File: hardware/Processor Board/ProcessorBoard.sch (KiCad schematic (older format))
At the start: 0 parts

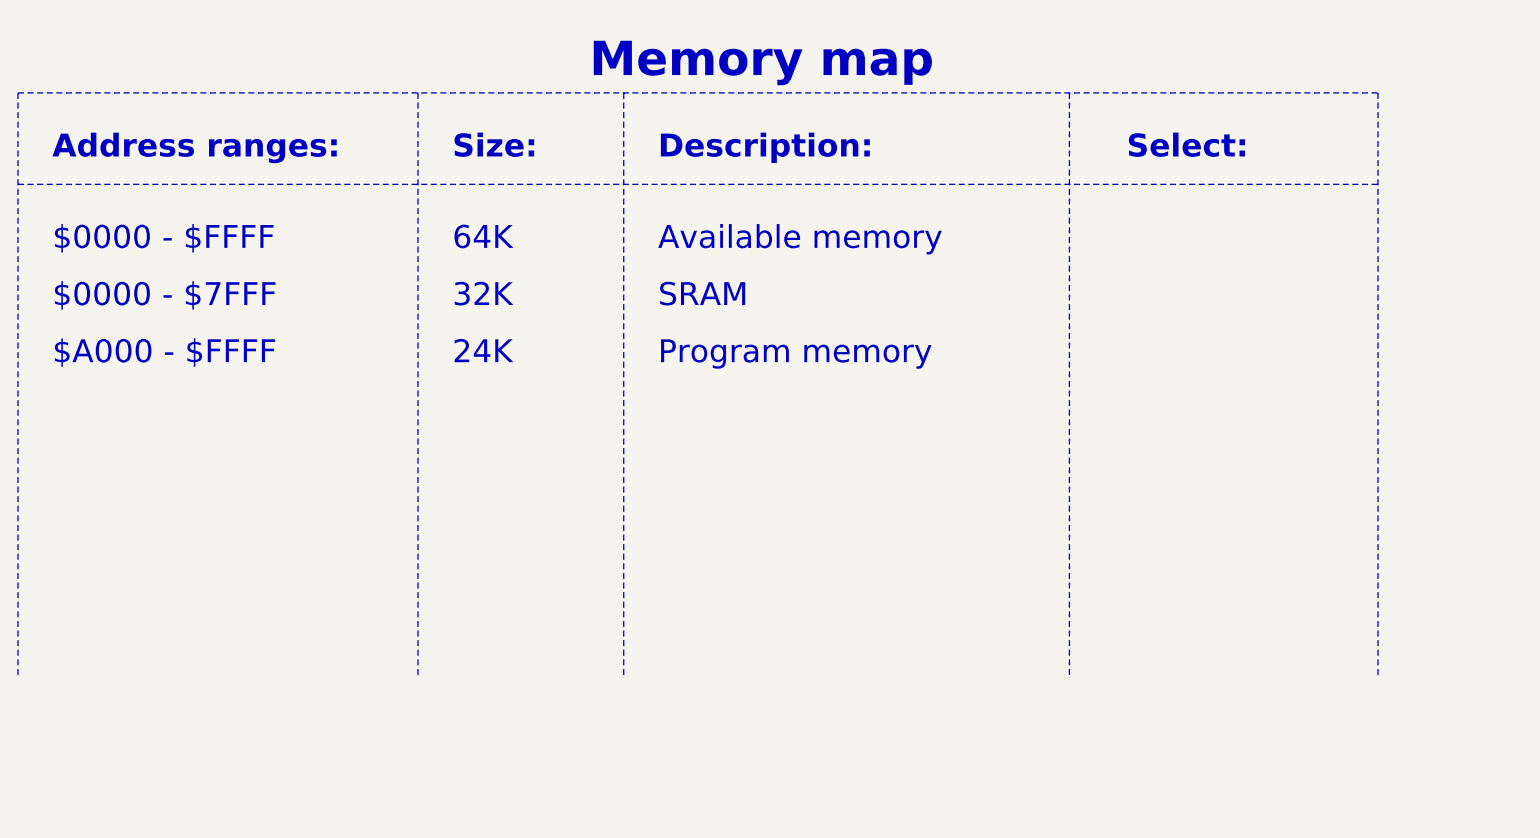
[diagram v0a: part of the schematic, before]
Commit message: Update processor board
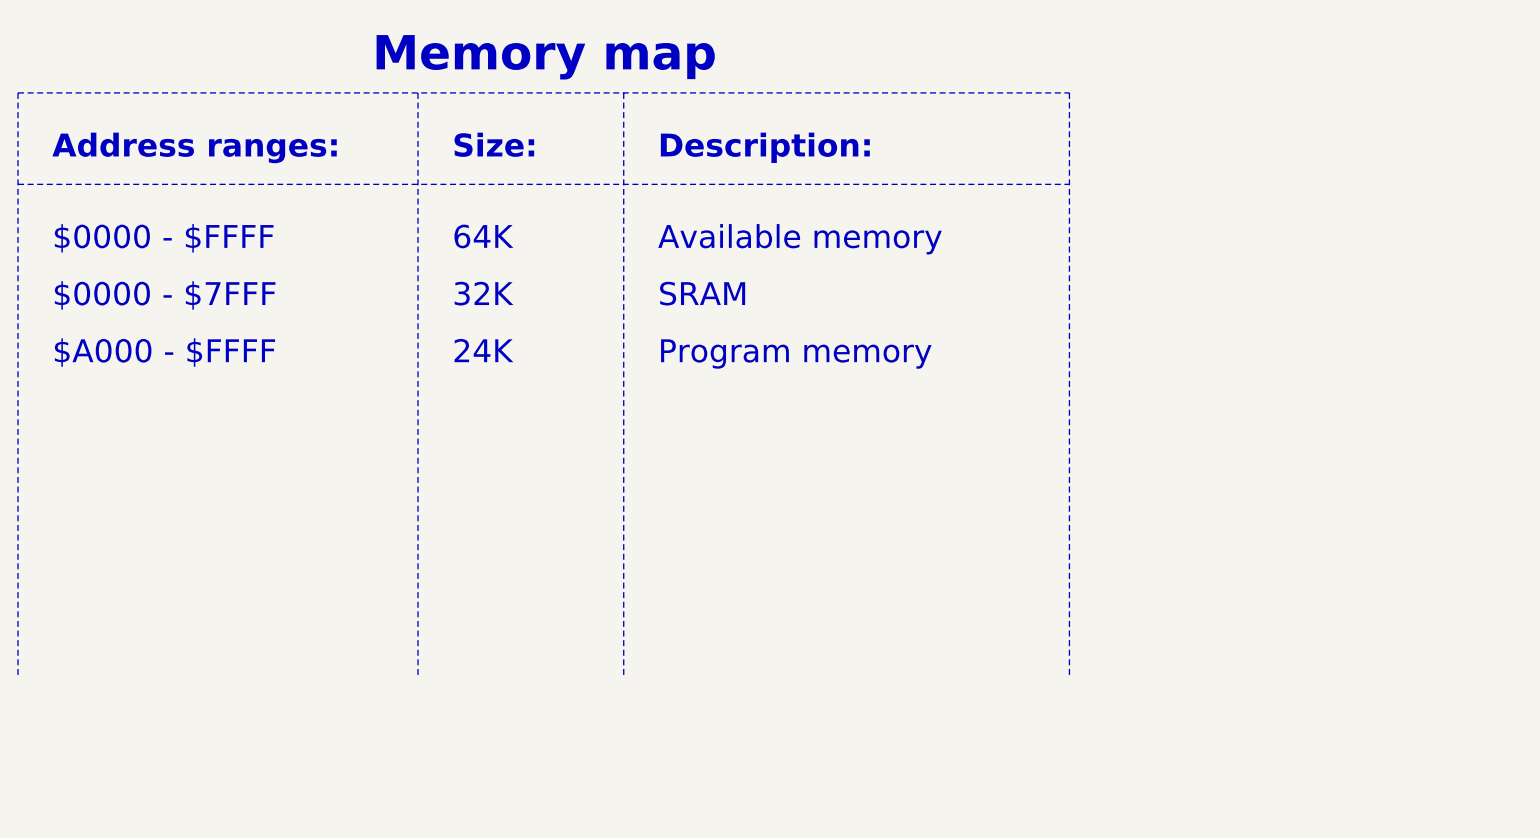
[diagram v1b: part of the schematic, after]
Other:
- note removed: "Select:"
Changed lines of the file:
@@
 Text Notes 3550 2100 0    100  ~ 0
 SRAM
-Text Notes 5600 1450 0    100  ~ 20
-Select:
 Wire Notes Line width 18 style solid
 	5350 1150 5350 3700
-Text Notes 3250 1100 0    150  ~ 30
+Text Notes 2300 1075 0    150  ~ 30
 Memory map
 Text Notes 900  1850 0    100  ~ 0
 $0000 - $FFFF\n
 Wire Notes Line width 18 style solid
-	750  1550 6700 1550
+	750  1550 5350 1550
 Wire Notes Line width 18 style solid
-	750  1150 6700 1150
-Wire Notes Line width 18 style solid
-	6700 1150 6700 3700
+	750  1150 5350 1150
 Wire Notes Line width 18 style solid
 	750  1150 750  3700
